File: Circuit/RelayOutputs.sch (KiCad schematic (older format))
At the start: 32 parts, among them K201 Meisei-m4-24h, K202 Meisei-m4-24h, K203 Meisei-m4-24h, K204 Meisei-m4-24h, K205 Meisei-m4-24h, K206 Meisei-m4-24h, K207 Meisei-m4-24h, K208 Meisei-m4-24h, Q201 Q_NPN_BCE, Q202 Q_NPN_BCE, Q203 Q_NPN_BCE, Q204 Q_NPN_BCE, Q205 Q_NPN_BCE, Q206 Q_NPN_BCE, Q207 Q_NPN_BCE, Q208 Q_NPN_BCE

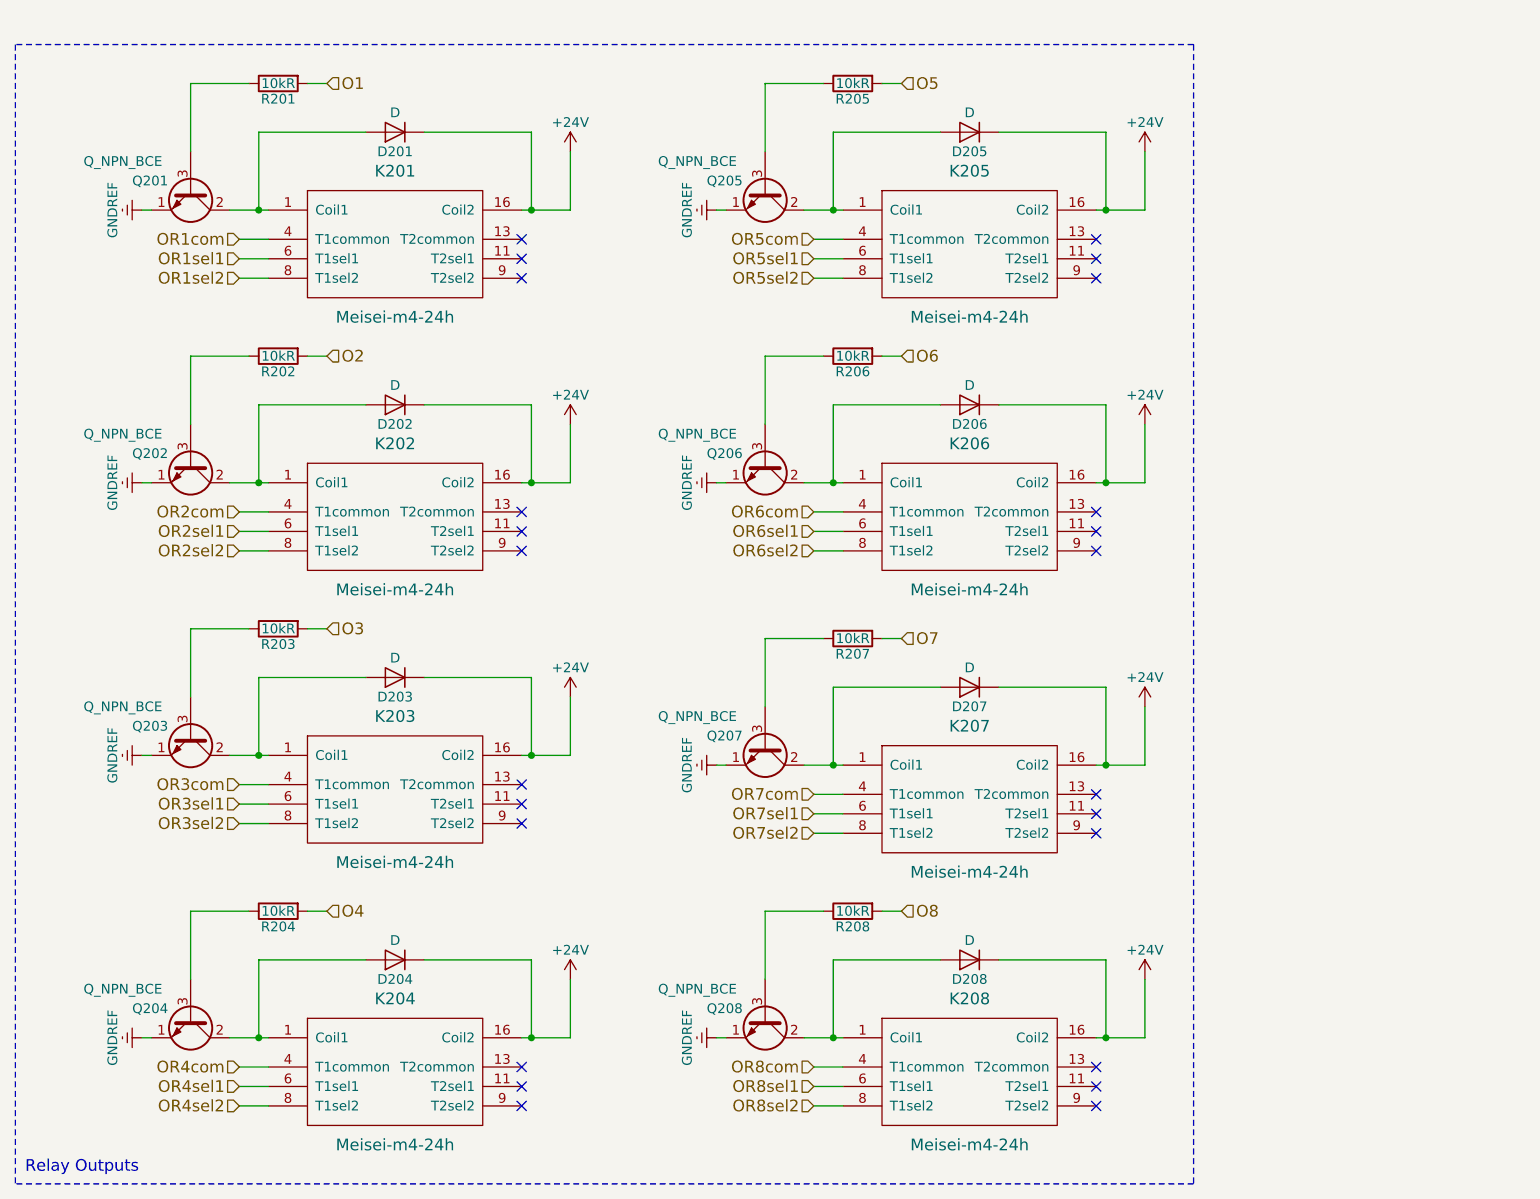
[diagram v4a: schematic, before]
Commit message: PCB. Pours mostly complete. Almost done?
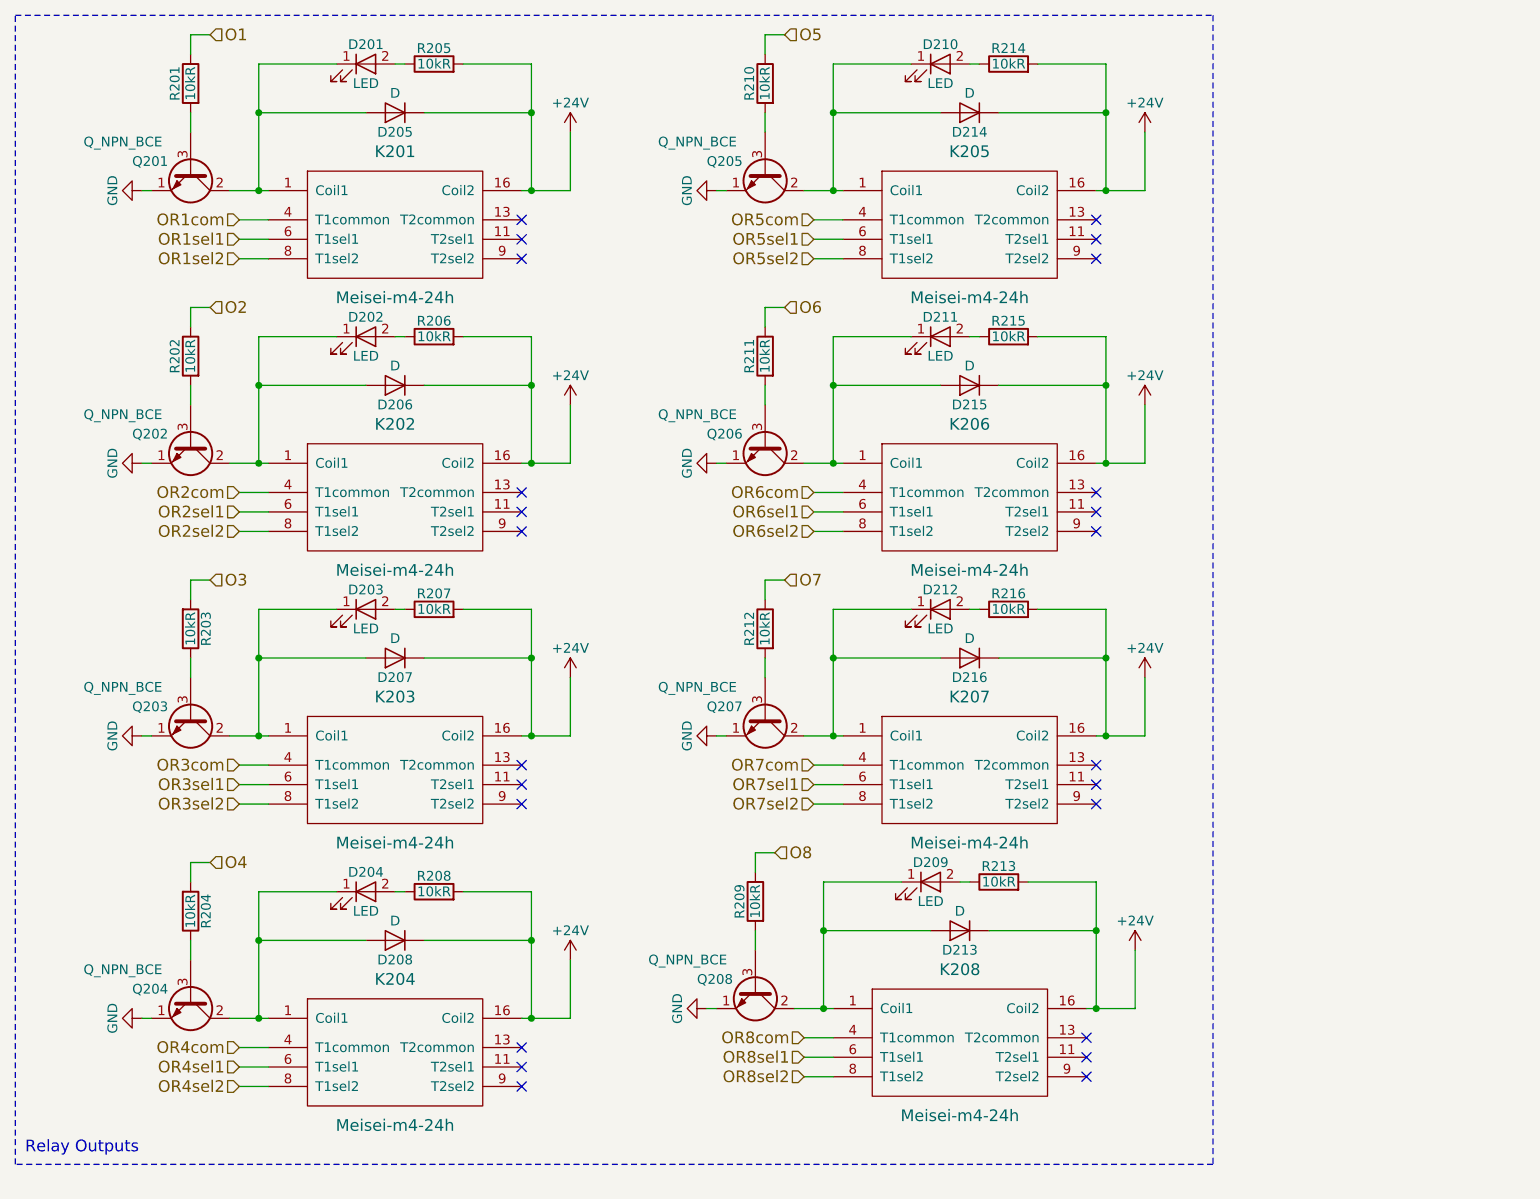
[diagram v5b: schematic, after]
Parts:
- added D201, D202, D203, D204, D209, D210, D211, D212: LED, Capacitors_SMD:C_0805, symbol LED
- added R205, R206, R207, R208, R213, R214, R215, R216: 10kR, Resistors_SMD:R_0805, symbol R
- renumbered D201 to D205, D202 to D206, D203 to D207, D204 to D208, D208 to D213, D205 to D214, D206 to D215, D207 to D216, R208 to R209, R205 to R210, R206 to R211, R207 to R212
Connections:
- net +24V: now also R205.2, R206.2, R207.2, R208.2, R213.2, R214.2, R215.2, R216.2
- net O1: now also R201.1; no longer R201.2
- net O2: now also R202.1; no longer R202.2
- net O5: now also R210.1; no longer R210.2
- net O6: now also R211.1; no longer R211.2
- net O7: now also R212.1; no longer R212.2
- net O8: now also R209.1; no longer R209.2
- net at D208.2 (A), K204.1 (Coil1), Q204.2 (C): now also D204.1 (K)
- net at D214.2 (A), K205.1 (Coil1), Q205.2 (C): now also D210.1 (K)
- net at Q205.3 (B): now also R210.2; no longer R210.1
- net at D215.2 (A), K206.1 (Coil1), Q206.2 (C): now also D211.1 (K)
- net at Q206.3 (B): now also R211.2; no longer R211.1
- net at D205.2 (A), K201.1 (Coil1), Q201.2 (C): now also D201.1 (K)
- net at Q201.3 (B): now also R201.2; no longer R201.1
- net at D206.2 (A), K202.1 (Coil1), Q202.2 (C): now also D202.1 (K)
- net at Q202.3 (B): now also R202.2; no longer R202.1
- net at D207.2 (A), K203.1 (Coil1), Q203.2 (C): now also D203.1 (K)
- net at D216.2 (A), K207.1 (Coil1), Q207.2 (C): now also D212.1 (K)
- net at Q207.3 (B): now also R212.2; no longer R212.1
- net at D213.2 (A), K208.1 (Coil1), Q208.2 (C): now also D209.1 (K)
- net at Q208.3 (B): now also R209.2; no longer R209.1
- net GNDREF renamed GND
- new net: D209.2 (A), R213.1
- new net: D212.2 (A), R216.1
- new net: D204.2 (A), R208.1
- new net: D203.2 (A), R207.1
- new net: D211.2 (A), R215.1
- new net: D210.2 (A), R214.1
- new net: D202.2 (A), R206.1
- new net: D201.2 (A), R205.1
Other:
- moved on the sheet: D205, D206, D207, D208, D213, D214, D215, D216, K201, K202, K203, K204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
